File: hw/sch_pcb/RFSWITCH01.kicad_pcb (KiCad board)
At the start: 2 copper layers, 40.1 x 40.1 mm, 45 parts, among them J1 HEADER_2x03_PARALLEL, J10 HEADER_2x01_PARALLEL, J2 SMA, J3 SMA, J4 HEADER_2x01_PARALLEL, J5 HEADER_2x01_PARALLEL, J6 HEADER_2x01_PARALLEL, J7 SMA, J8 SMA, J9 HEADER_2x01_PARALLEL, M1 HOLE, M2 HOLE, M3 HOLE, M4 HOLE, U1 TPS22945DCKR, U2 PE4259, U3 SPF5189Z, U4 PE4259

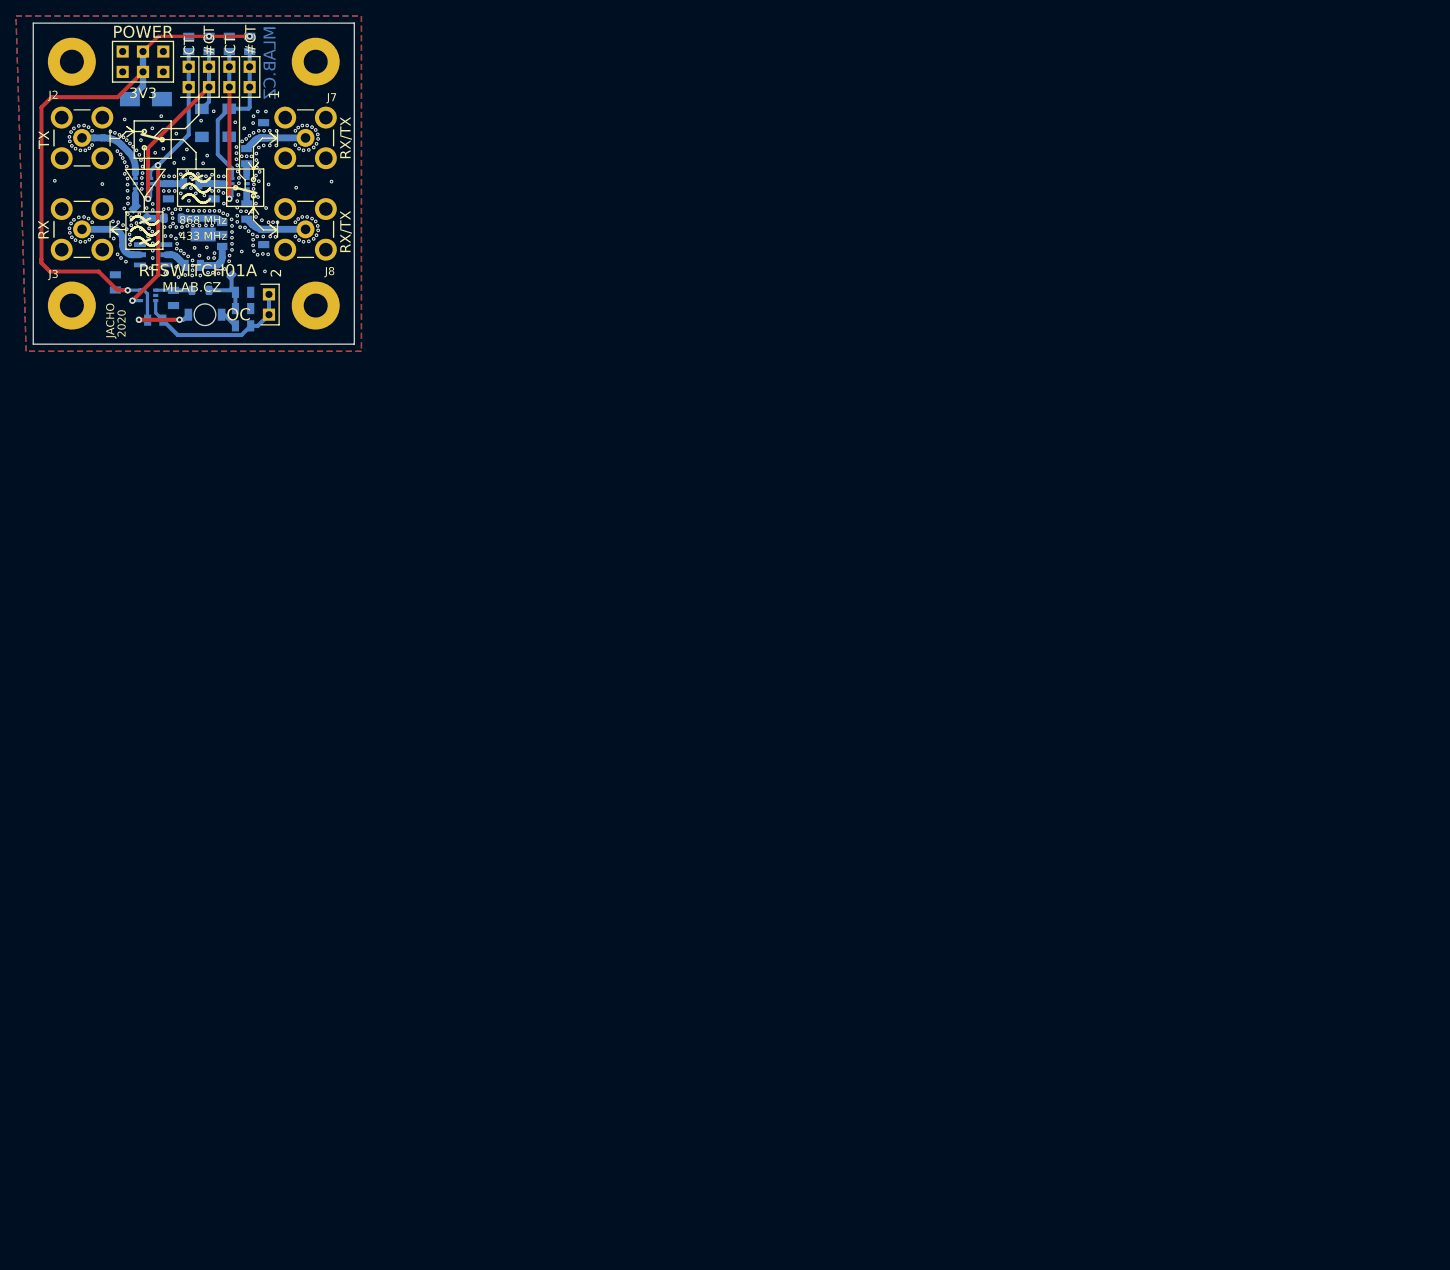
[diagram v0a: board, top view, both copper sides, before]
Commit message: update kicad
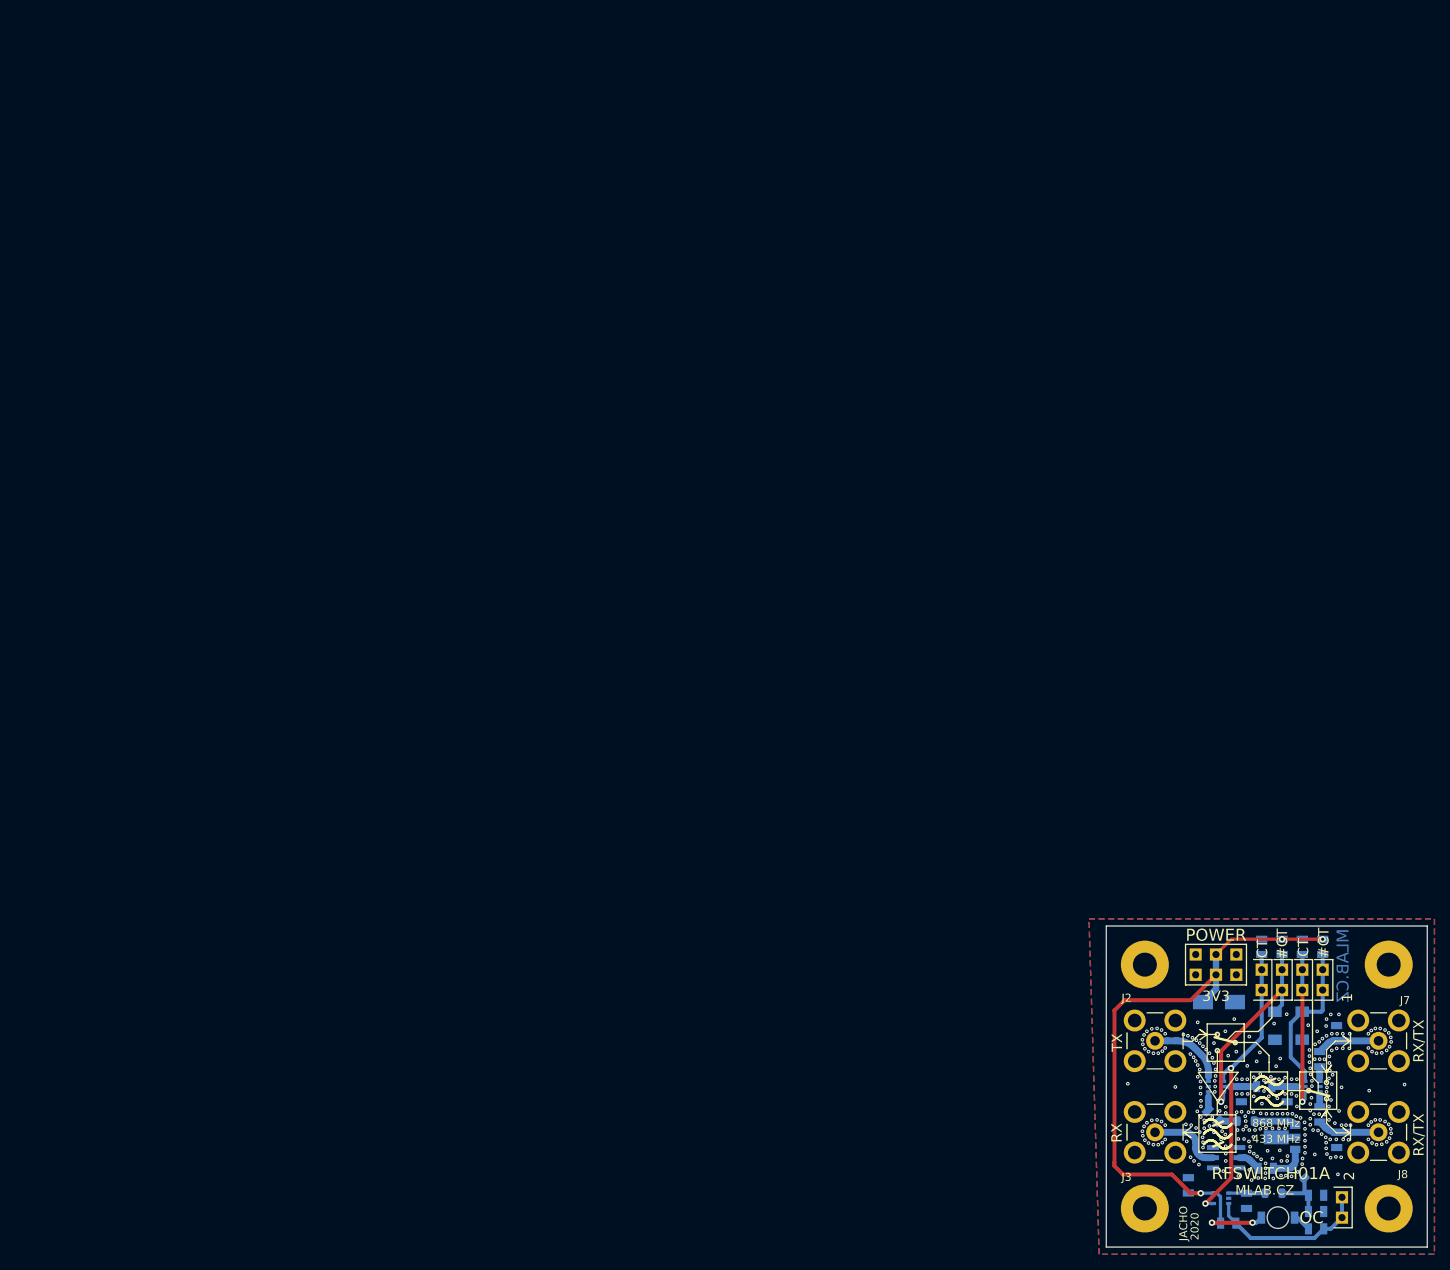
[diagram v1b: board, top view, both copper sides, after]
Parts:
- moved C10 175.3 mm to (157.0, 93.5)
- moved C5 175.3 mm to (154.3, 102.8)
- moved C7 175.3 mm to (161.1, 96.0)
- moved C8 175.3 mm to (147.7, 96.2)
- moved C9 175.3 mm to (151.3, 93.5)
- moved D2 175.3 mm to (158.9, 84.9)
- moved D3 175.3 mm to (155.5, 85.0)
- moved FL1 175.3 mm to (149.4, 101.4)
- moved J1 175.3 mm to (148.1, 77.3)
- moved J3 175.3 mm to (140.5, 98.3)
- moved J8 175.3 mm to (168.4, 98.3)
- moved L2 175.3 mm to (158.4, 103.3)
- moved L5 175.3 mm to (163.2, 99.2)
- moved L6 175.3 mm to (154.1, 92.5)
- moved M1 175.3 mm to (169.7, 77.3)
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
